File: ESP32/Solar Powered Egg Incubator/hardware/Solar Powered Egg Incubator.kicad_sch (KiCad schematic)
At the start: 102 parts, among them J1 FAN, J2 SPINNER, J23 USB_C Conn, J3 BMS, J4 RTC, J42 Ultra Sonic, J47 SCREEN, J5 AHT20, J6 HUMIDIFIER, J7 HEATER, J8 LEVELS, K4 RELAY, K5 RELAY, K6 RELAY, Q2 UMH3N, Q9 TIP41, SW4 RESET, SW5 FLASH, SW6 RotaryEncoder, U1 LM2596S-3.3V, U3 LM2596S-5V, U5 AMS1117-3.3, U7 ESP32-WROOM, U8 CH340C, Y2 12MHz

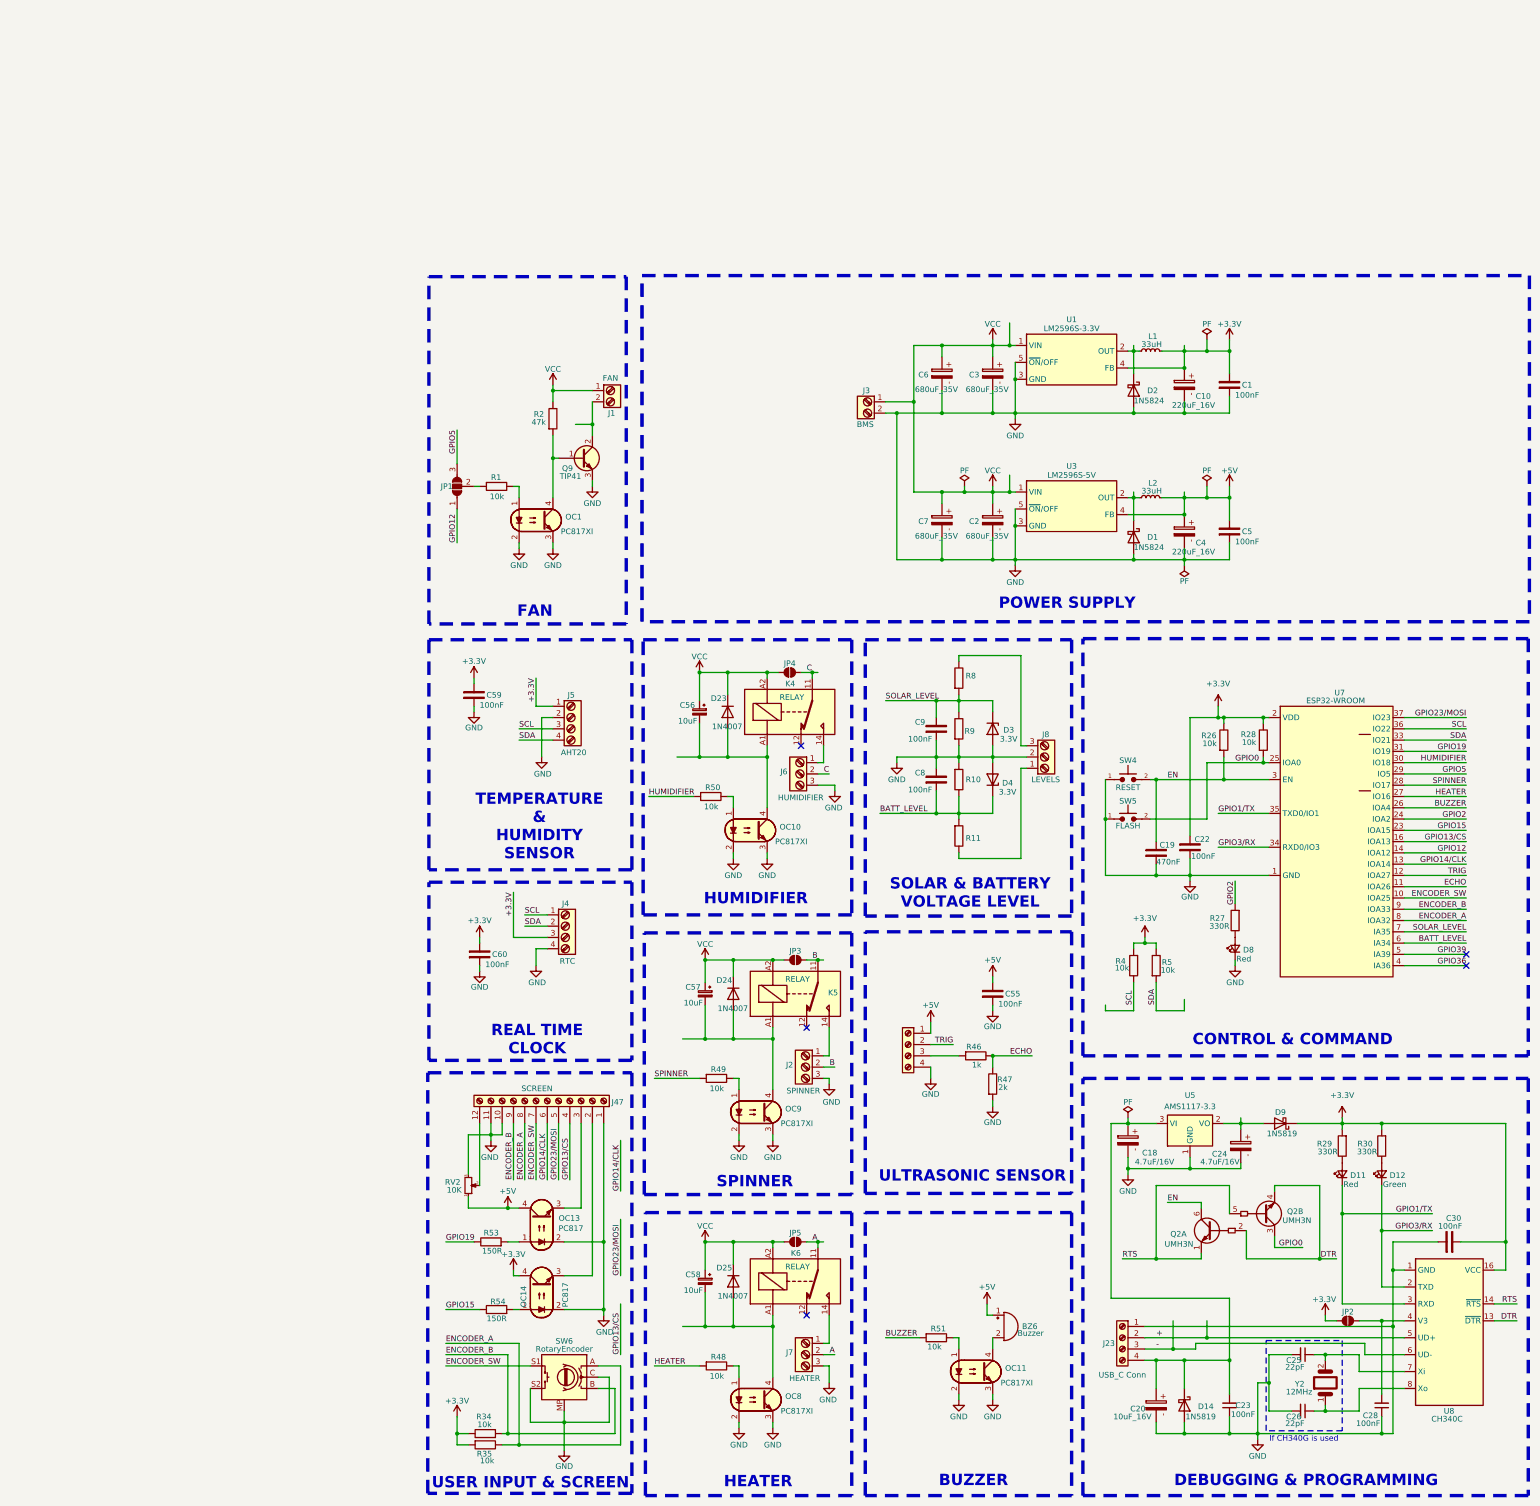
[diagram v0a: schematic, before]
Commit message: sync updates
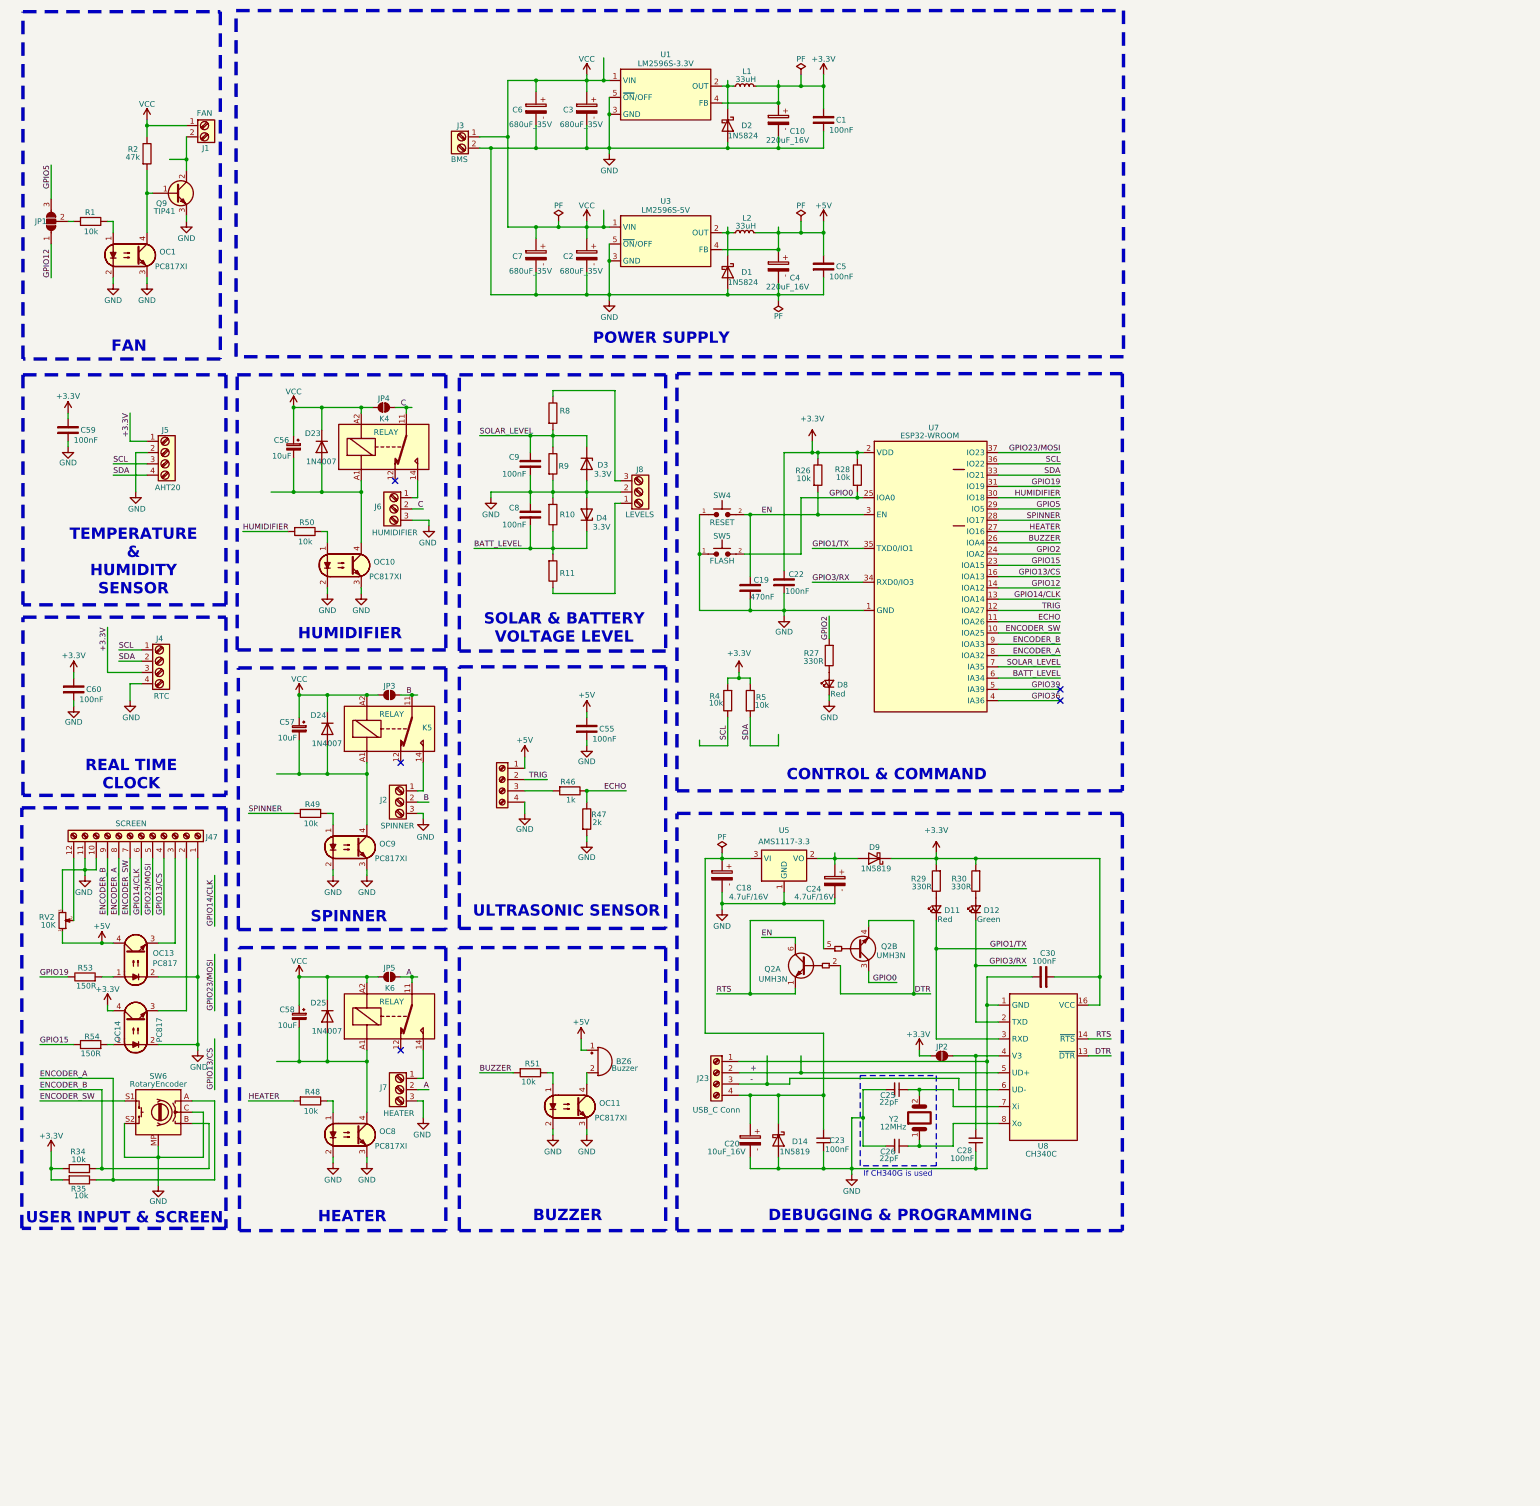
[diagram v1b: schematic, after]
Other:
- moved on the sheet: BZ6, C1, C10, C18, C19, C2, C20, C22, C23, C24, C25, C26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
